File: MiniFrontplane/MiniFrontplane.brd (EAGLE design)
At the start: 95.7 x 39.4 mm, 17 parts, among them IC2 74ACT14N, U1 MCP130SOT

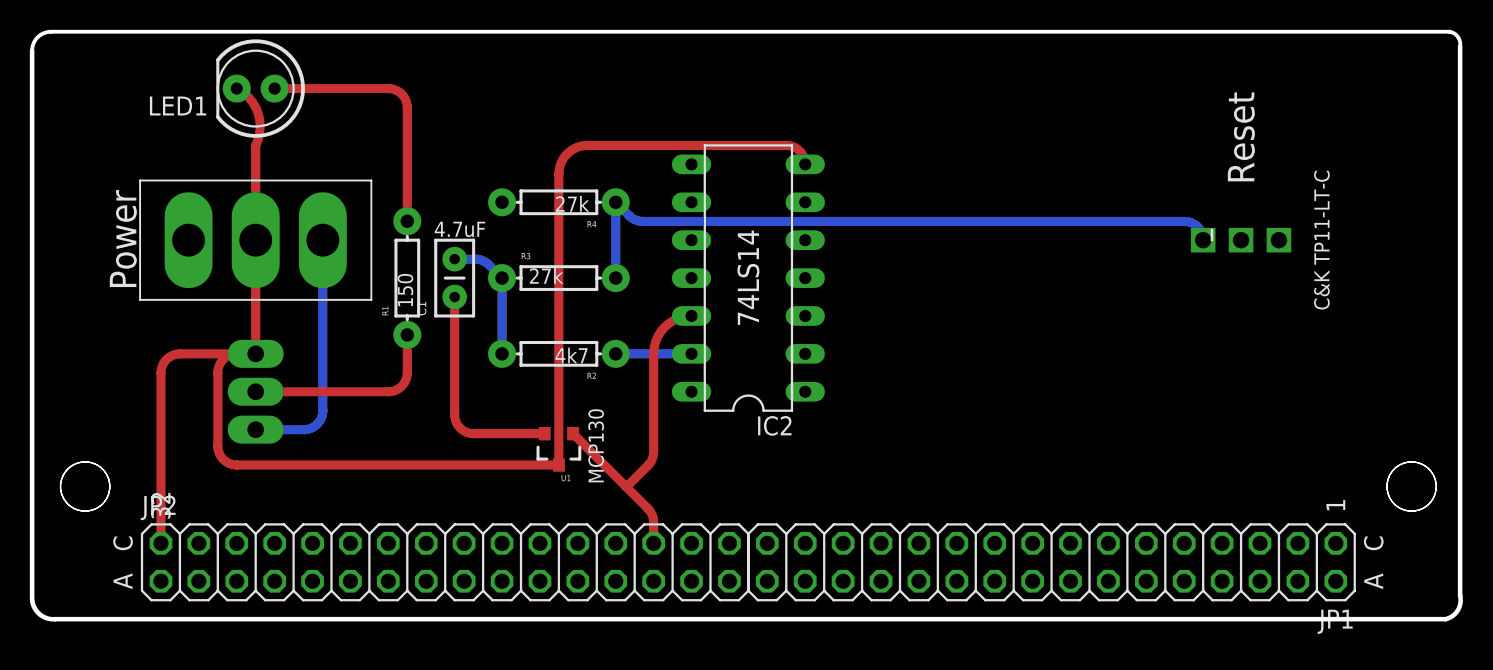
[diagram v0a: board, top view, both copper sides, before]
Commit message: Fixed a whole lot of shit
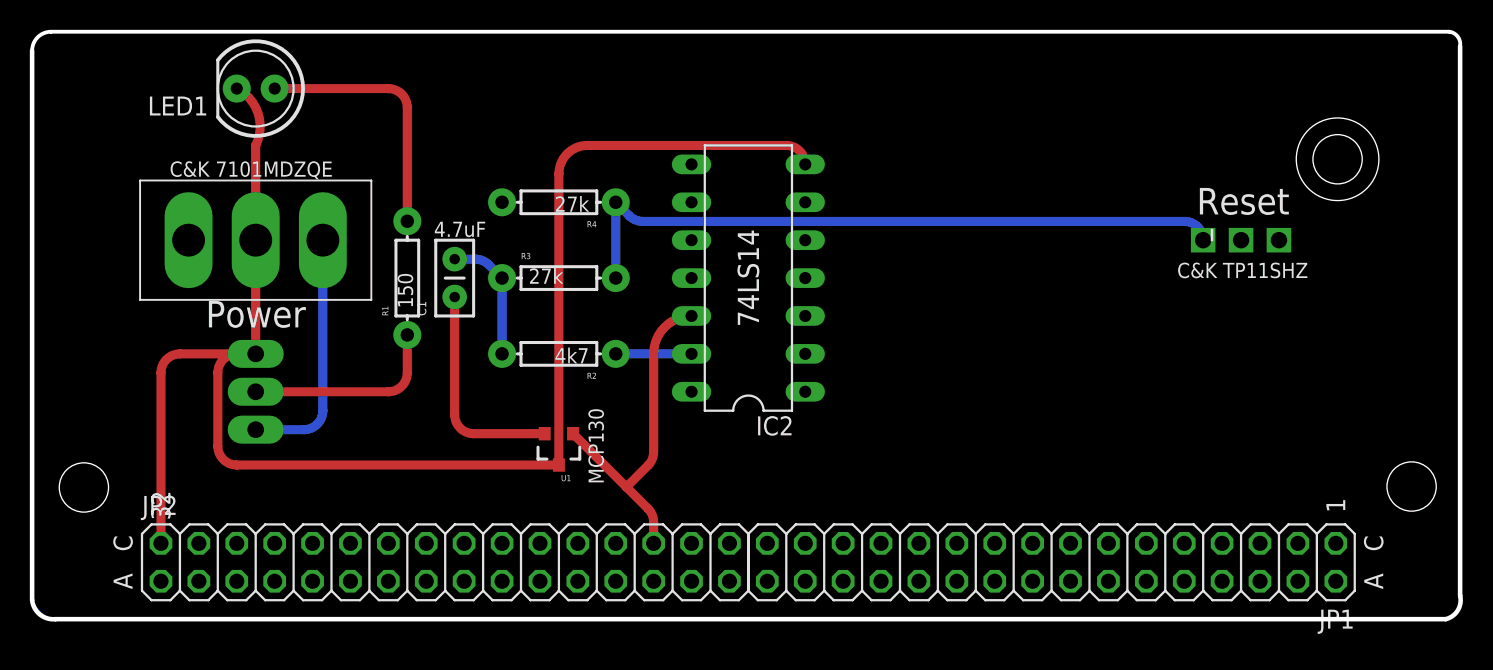
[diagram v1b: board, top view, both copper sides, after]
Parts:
- removed U$10, U$11, U$12: (no value), SparkFun-Electromechanical:STAND-OFF
- added U$22, U$4: (no value), SparkFun-Electromechanical:STAND-OFF
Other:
- board text added: "C&K 7101MDZQE"
- board text added: "C&K TP11SHZ"
- board text removed: "C&K TP11-LT-C"
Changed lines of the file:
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@@
 <text x="92.2868375" y="6.515021875" size="1.27" layer="21" font="vector" ratio="15" rot="R90" align="center">C</text>
 <text x="92.2868375" y="3.975021875" size="1.27" layer="21" font="vector" ratio="15" rot="R90" align="center">A</text>
-<text x="83.3968375" y="30.560415625" size="1.778" layer="21" font="vector" ratio="15" rot="R90" align="center-left">Reset</text>
-<text x="8.4668375" y="26.835021875" size="1.778" layer="21" font="vector" ratio="15" rot="R90" align="center">Power</text>
+<text x="83.536384375" y="29.4472375" size="1.778" layer="21" font="vector" ratio="15" rot="R180" align="center">Reset</text>
+<text x="17.360978125" y="21.8780375" size="1.778" layer="21" font="vector" ratio="15" rot="R180" align="center">Power</text>
 <text x="50.3768375" y="24.295021875" size="1.4224" layer="21" font="vector" ratio="15" rot="R90" align="center">74LS14</text>
 <text x="32.810834375" y="27.564409375" size="1.016" layer="21" font="vector" ratio="15" rot="R180" align="center-left">4.7uF</text>
 <text x="40.682496875" y="13.0343625" size="1.016" layer="21" font="vector" ratio="15" rot="R90" align="bottom-center">MCP130</text>
-<text x="89.323546875" y="26.835021875" size="1.016" layer="21" font="vector" ratio="15" rot="R90" align="bottom-center">C&amp;K TP11-LT-C</text>
+<text x="83.502578125" y="25.315546875" size="1.016" layer="21" font="vector" ratio="15" rot="R180" align="bottom-center">C&amp;K TP11SHZ</text>
 <rectangle x1="81.02549375" y1="27.0947375" x2="81.8713125" y2="27.2639" layer="21" rot="R90"/>
+<text x="11.5824" y="31.0896" size="1.016" layer="21" font="vector" ratio="15">C&amp;K 7101MDZQE</text>
+<hole x="89.8652" y="32.258" drill="5.5372"/>
 </plain>
 <attributes>
@@
 <elements>
 <element name="U$9" library="SparkFun-Electromechanical" package="STAND-OFF" value="" x="94.8268375" y="10.325021875" rot="MR90"/>
-<element name="U$10" library="SparkFun-Electromechanical" package="STAND-OFF" value="" x="5.9268375" y="10.325021875" rot="MR90"/>
-<element name="U$11" library="SparkFun-Electromechanical" package="STAND-OFF" value="" x="94.8268375" y="10.325021875" rot="MR90"/>
-<element name="U$12" library="SparkFun-Electromechanical" package="STAND-OFF" value="" x="5.9268375" y="10.325021875" rot="MR90"/>
 <element name="JP2" library="pinhead" package="2X16" value="" x="30.0568375" y="5.245021875"/>
 <element name="JP1" library="pinhead" package="2X16" value="" x="70.6968375" y="5.245021875" rot="R180"/>
@@
 <element name="U$2" library="Benchoff" package="MINITACT" value="MINITACT" x="83.3968375" y="26.835021875" rot="R270"/>
 <element name="IC2" library="74xx-eu" package="DIL14" value="74ACT14N" x="50.3768375" y="24.295021875" rot="R90"/>
+<element name="U$4" library="SparkFun-Electromechanical" package="STAND-OFF" value="" x="5.842" y="10.2616" rot="MR90"/>
+<element name="U$22" library="SparkFun-Electromechanical" package="STAND-OFF" value="" x="89.8652" y="32.258" rot="MR270"/>
 </elements>
 <signals>
